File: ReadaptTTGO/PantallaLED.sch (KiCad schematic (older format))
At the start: 1 part

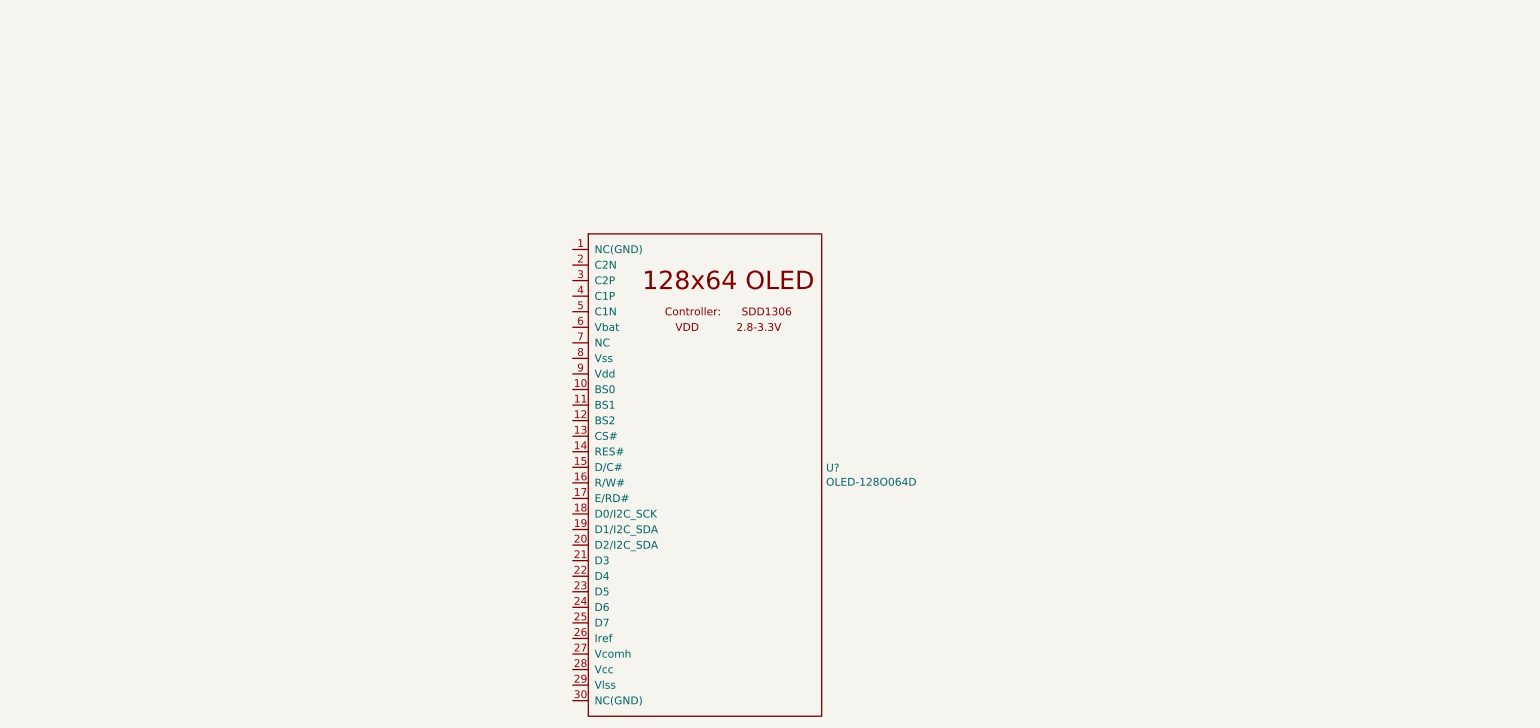
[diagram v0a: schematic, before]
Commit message: Primer aproximacion.
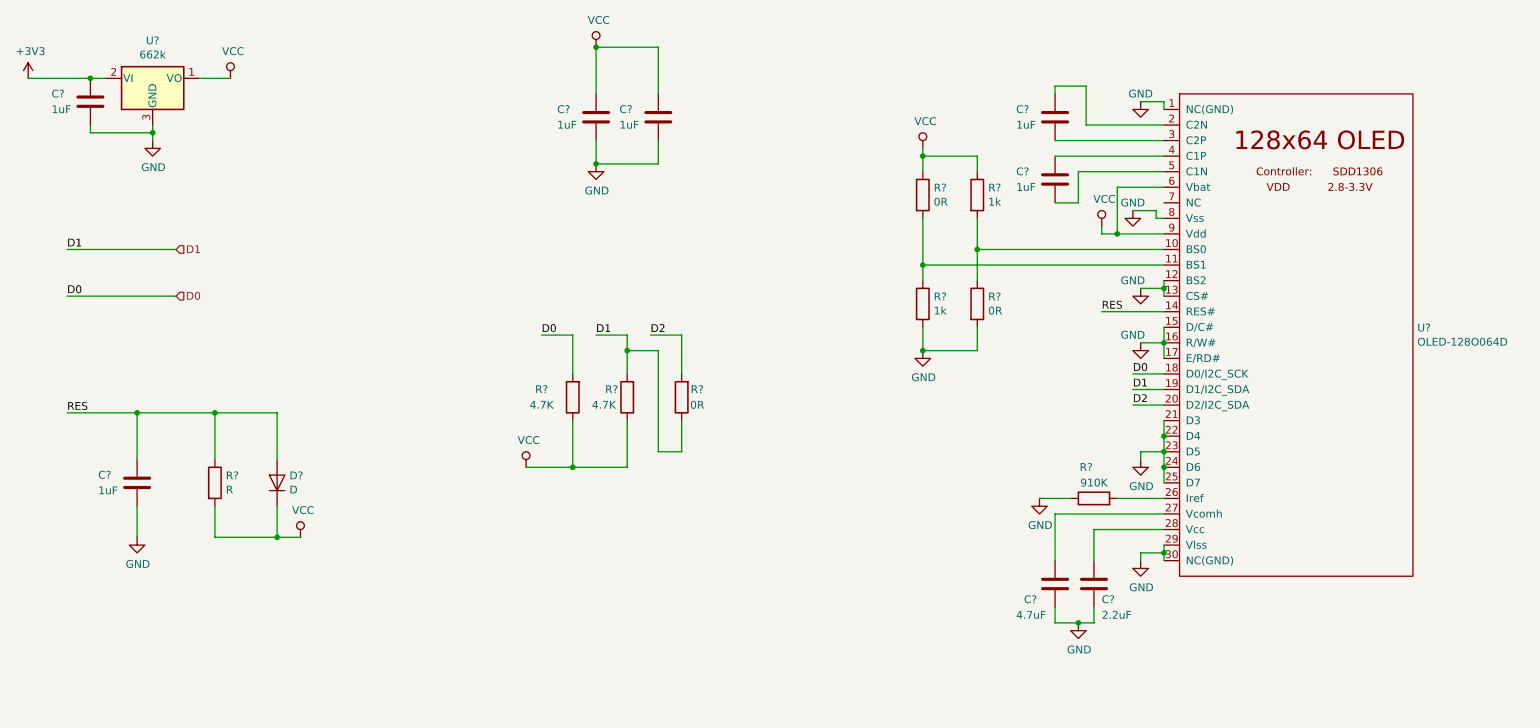
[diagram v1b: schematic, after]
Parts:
- added C? (x6): 1uF, symbol Device:C
- added C?: 4.7uF, symbol Device:C
- added C?: 2.2uF, symbol Device:C
- added D?: D, symbol Device:D
- added R? (x3): 0R, symbol Device:R
- added R? (x2): 1k, symbol Device:R
- added R?: 910K, symbol Device:R
- added R? (x2): 4.7K, symbol Device:R
- added R?: R, symbol Device:R
- added U?: 662k, Package_TO_SOT_SMD:SOT-23, symbol Regulator_Linear:LM3480-3.3
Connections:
- net GND: now reaches U?.1 (NC(GND))
- net GND: now also U?.12 (BS2), U?.13 (CS#), U?.15 (D/C#), U?.16 (R/W#), U?.17 (E/RD#), U?.21 (D3), U?.22 (D4), U?.23 (D5), U?.24 (D6), U?.25 (D7), U?.29 (Vlss), U?.30 (NC(GND)), U?.8 (Vss), C?.2, C?.2, C?.2, C?.2, C?.2, C?.2, R?.1, R?.2, R?.2, U?.3 (GND)
- net at U?.10 (BS0): now also R?.1, R?.2
- net at U?.11 (BS1): now also R?.1, R?.2
- net RES: now reaches U?.14 (RES#)
- net RES: now also C?.1, D?.2 (A), R?.1
- net D0: now reaches U?.18 (D0/I2C_SCK)
- net D0: now also R?.2
- net D1: now reaches U?.19 (D1/I2C_SDA)
- net D1: now also R?.1, R?.2
- net at U?.2 (C2N): now also C?.1
- net D2: now reaches U?.20 (D2/I2C_SDA)
- net D2: now also R?.2
- net at U?.26 (Iref): now also R?.2
- net at U?.27 (Vcomh): now also C?.1
- net at U?.28 (Vcc): now also C?.1
- net at U?.3 (C2P): now also C?.2
- net at U?.4 (C1P): now also C?.1
- net at U?.5 (C1N): now also C?.2
- net VCC: now reaches U?.6 (Vbat)
- net VCC: now also U?.9 (Vdd), C?.1, C?.1, D?.1 (K), R?.1, R?.1, R?.1, R?.1, R?.2, U?.1 (VO)
- new net +3V3: C?.1, U?.2 (VI)
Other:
- moved on the sheet: U?
